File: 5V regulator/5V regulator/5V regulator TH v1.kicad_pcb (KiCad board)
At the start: 2 copper layers, 48.3 x 29.2 mm, 14 parts, among them J1 9V Vhod, J2 5V Izhod, U1 LM7805

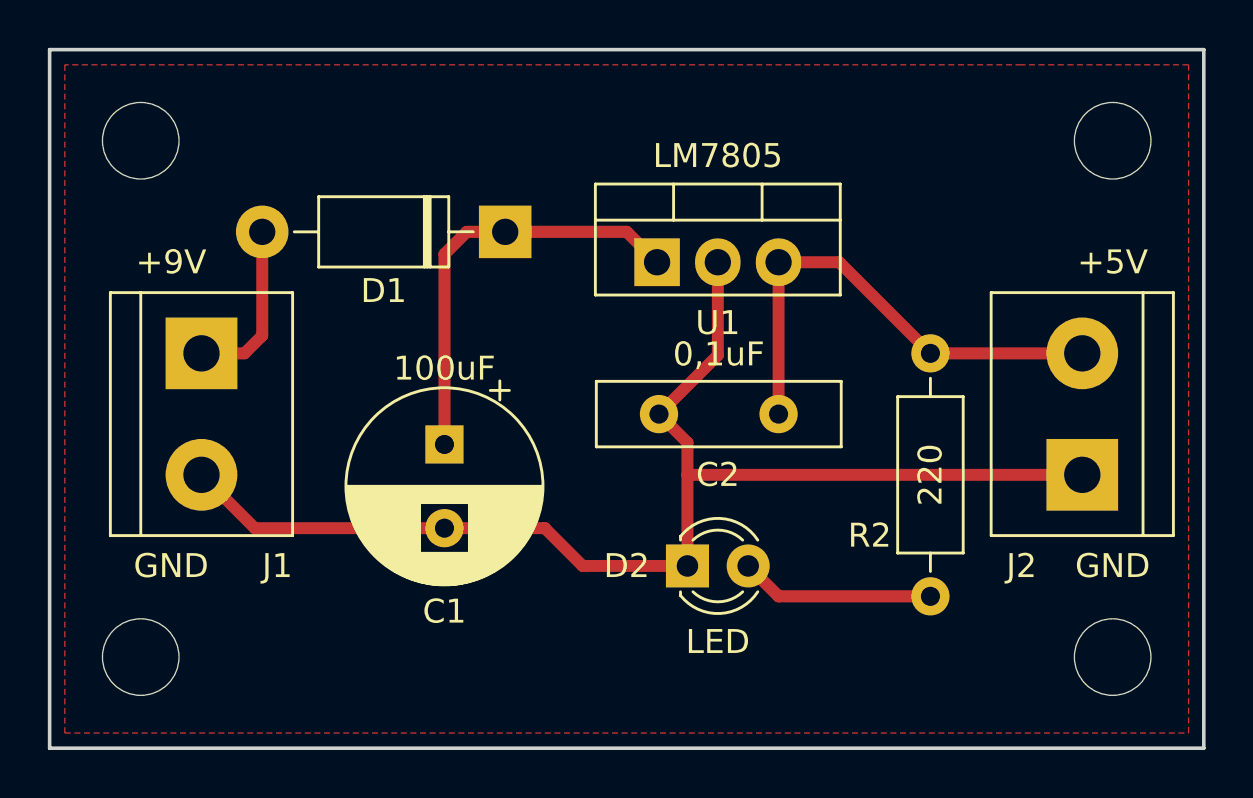
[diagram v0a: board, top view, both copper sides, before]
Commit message: update doma
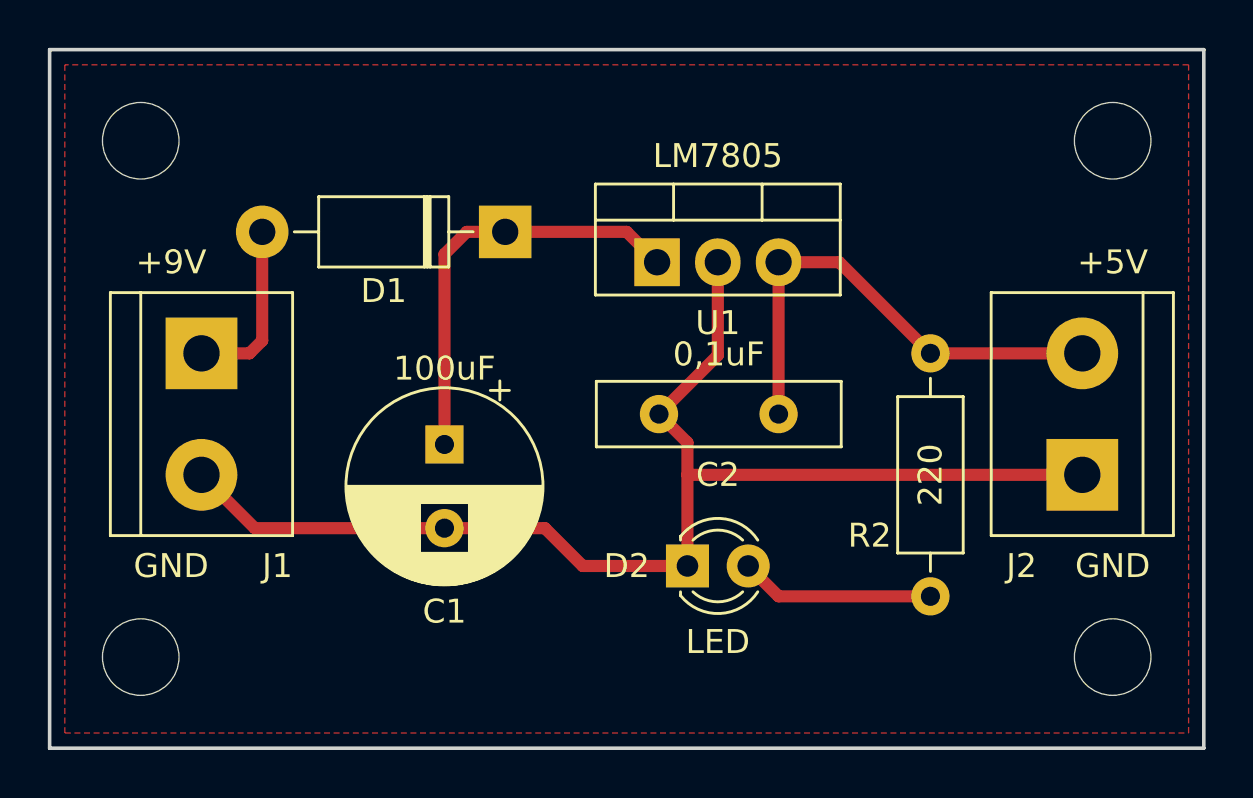
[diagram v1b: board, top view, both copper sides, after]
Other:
- net class PWR_TRACK removed
